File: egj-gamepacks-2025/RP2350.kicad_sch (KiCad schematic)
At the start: 41 parts, among them J3 SM03B-SRSS-TB, SW1 SW_Push, SW2 SW_Push, U1 W25Q128JVS, U2 DNF, U4 RP2350_80QFN, U5 USBLC6-2P6, Y1 ABM8-272-T3

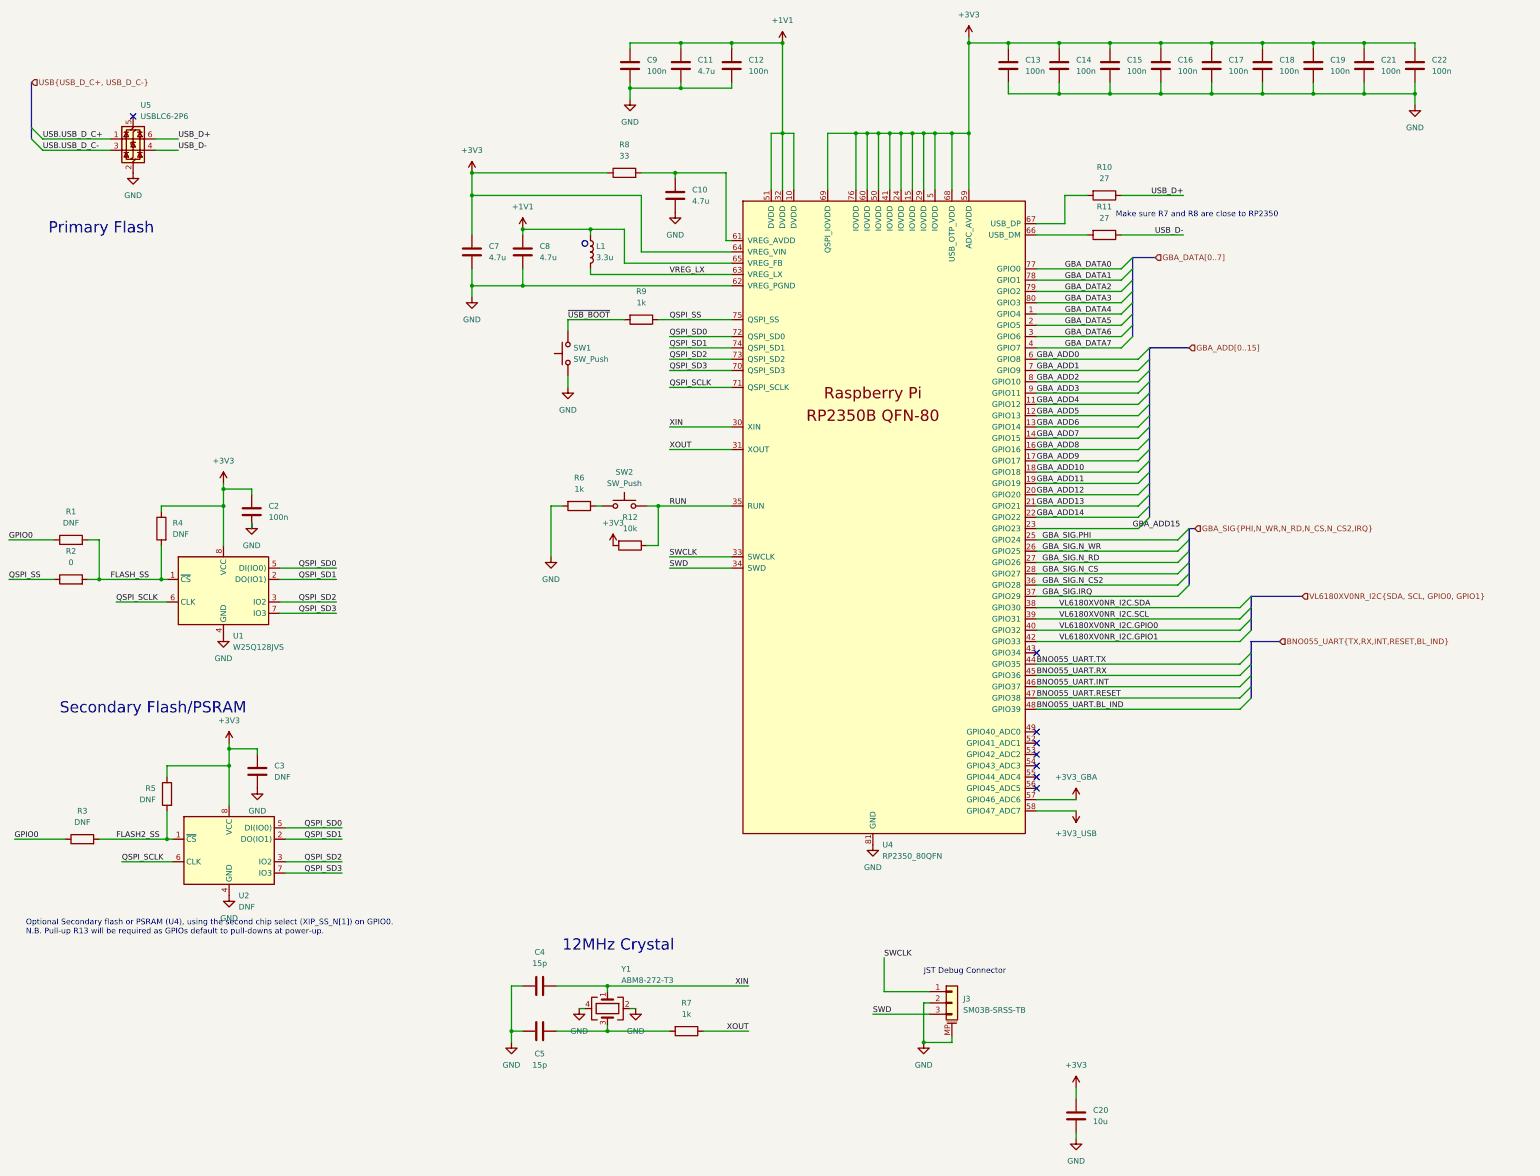
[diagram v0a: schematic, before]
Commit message: Update
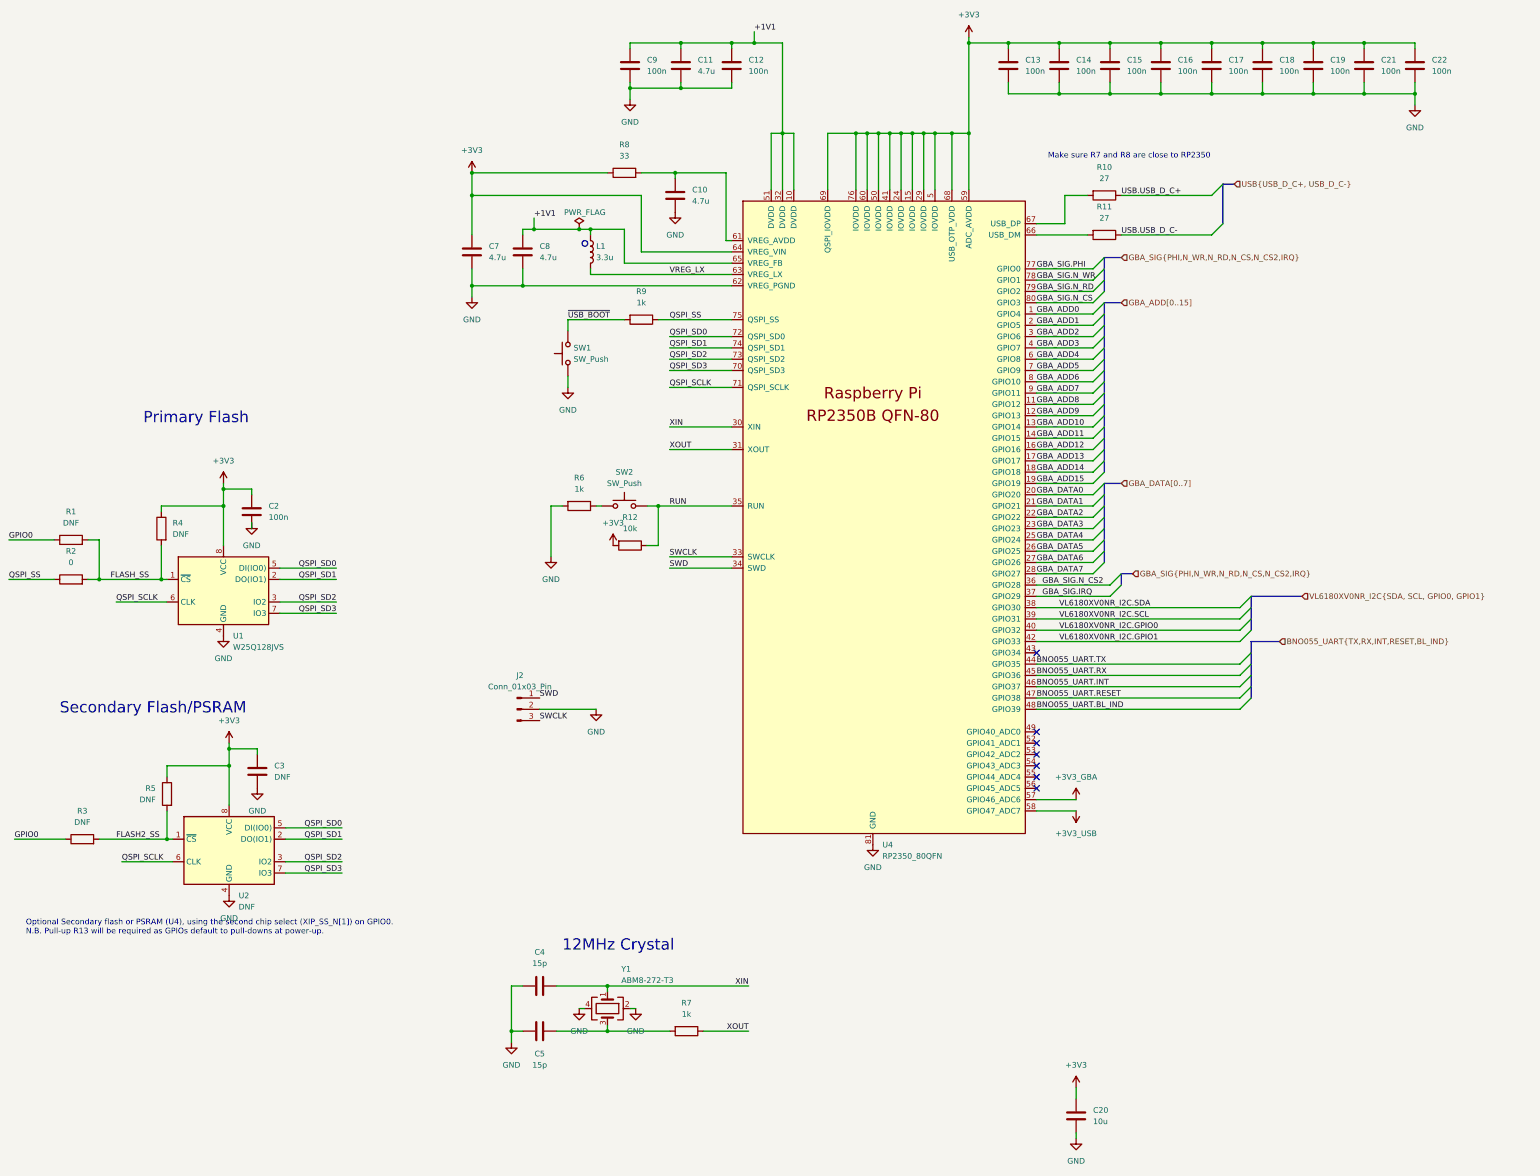
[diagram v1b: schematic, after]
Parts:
- removed J3: SM03B-SRSS-TB, Connector_JST:JST_SH_SM03B-SRSS-TB_1x03-1MP_P1.00mm_Horizontal, symbol Connector_Generic_MountingPin:Conn_01x03_MountingPin
- removed U5: USBLC6-2P6, Package_TO_SOT_SMD:SOT-666, symbol Power_Protection:USBLC6-2P6
- added J2: Conn_01x03_Pin, Connector_PinHeader_2.54mm:PinHeader_1x03_P2.54mm_Horizontal, symbol Connector:Conn_01x03_Pin
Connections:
- net USB_D+ is gone; now on net USB.USB_D_C+: R10.1
- net USB_D- is gone; now on net USB.USB_D_C-: R11.1
- net GBA_ADD0: now also U4.1 (GPIO4); no longer U4.6 (GPIO8)
- net GBA_ADD1: now also U4.2 (GPIO5); no longer U4.7 (GPIO9)
- net GBA_ADD10: now also U4.13 (GPIO14); no longer U4.18 (GPIO18)
- net GBA_ADD11: now also U4.14 (GPIO15); no longer U4.19 (GPIO19)
- net GBA_ADD12: now also U4.16 (GPIO16); no longer U4.20 (GPIO20)
- net GBA_ADD13: now also U4.17 (GPIO17); no longer U4.21 (GPIO21)
- net GBA_ADD14: now also U4.18 (GPIO18); no longer U4.22 (GPIO22)
- net GBA_ADD15: now also U4.19 (GPIO19); no longer U4.23 (GPIO23)
- net GBA_ADD2: now also U4.3 (GPIO6); no longer U4.8 (GPIO10)
- net GBA_ADD3: now also U4.4 (GPIO7); no longer U4.9 (GPIO11)
- net GBA_ADD4: now also U4.6 (GPIO8); no longer U4.11 (GPIO12)
- net GBA_ADD5: now also U4.7 (GPIO9); no longer U4.12 (GPIO13)
- net GBA_ADD6: now also U4.8 (GPIO10); no longer U4.13 (GPIO14)
- net GBA_ADD7: now also U4.9 (GPIO11); no longer U4.14 (GPIO15)
- net GBA_ADD8: now also U4.11 (GPIO12); no longer U4.16 (GPIO16)
- net GBA_ADD9: now also U4.12 (GPIO13); no longer U4.17 (GPIO17)
- net GBA_DATA0: now also U4.20 (GPIO20); no longer U4.77 (GPIO0)
- net GBA_DATA1: now also U4.21 (GPIO21); no longer U4.78 (GPIO1)
- net GBA_DATA2: now also U4.22 (GPIO22); no longer U4.79 (GPIO2)
- net GBA_DATA3: now also U4.23 (GPIO23); no longer U4.80 (GPIO3)
- net GBA_DATA4: now also U4.25 (GPIO24); no longer U4.1 (GPIO4)
- net GBA_DATA5: now also U4.26 (GPIO25); no longer U4.2 (GPIO5)
- net GBA_DATA6: now also U4.27 (GPIO26); no longer U4.3 (GPIO6)
- net GBA_DATA7: now also U4.28 (GPIO27); no longer U4.4 (GPIO7)
- net GBA_SIG.N_CS: now also U4.80 (GPIO3); no longer U4.28 (GPIO27)
- net GBA_SIG.N_RD: now also U4.79 (GPIO2); no longer U4.27 (GPIO26)
- net GBA_SIG.N_WR: now also U4.78 (GPIO1); no longer U4.26 (GPIO25)
- net GBA_SIG.PHI: now also U4.77 (GPIO0); no longer U4.25 (GPIO24)
- net GND: now also J2.2 (Pin_2)
- net SWCLK: now also J2.3 (Pin_3)
- net SWD: now also J2.1 (Pin_1)
- no-connect marks 8 -> 7
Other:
- note removed: "JST Debug Connector"
